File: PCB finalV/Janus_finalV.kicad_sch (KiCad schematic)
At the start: 37 parts, among them J1 Conn_01x02, J10 Conn_01x02, J11 Conn_01x04, J14 Conn_01x04, J15 Conn_01x04, J2 Conn_01x04, J3 BU33SD5WG-TR, J4 R-78B5.0-2.0, J5 Conn_01x03, J6 Conn_01x03, J7 Conn_ST_STDC14, J8 Conn_01x06, J9 Conn_01x02, U1 STM32L552CCTx

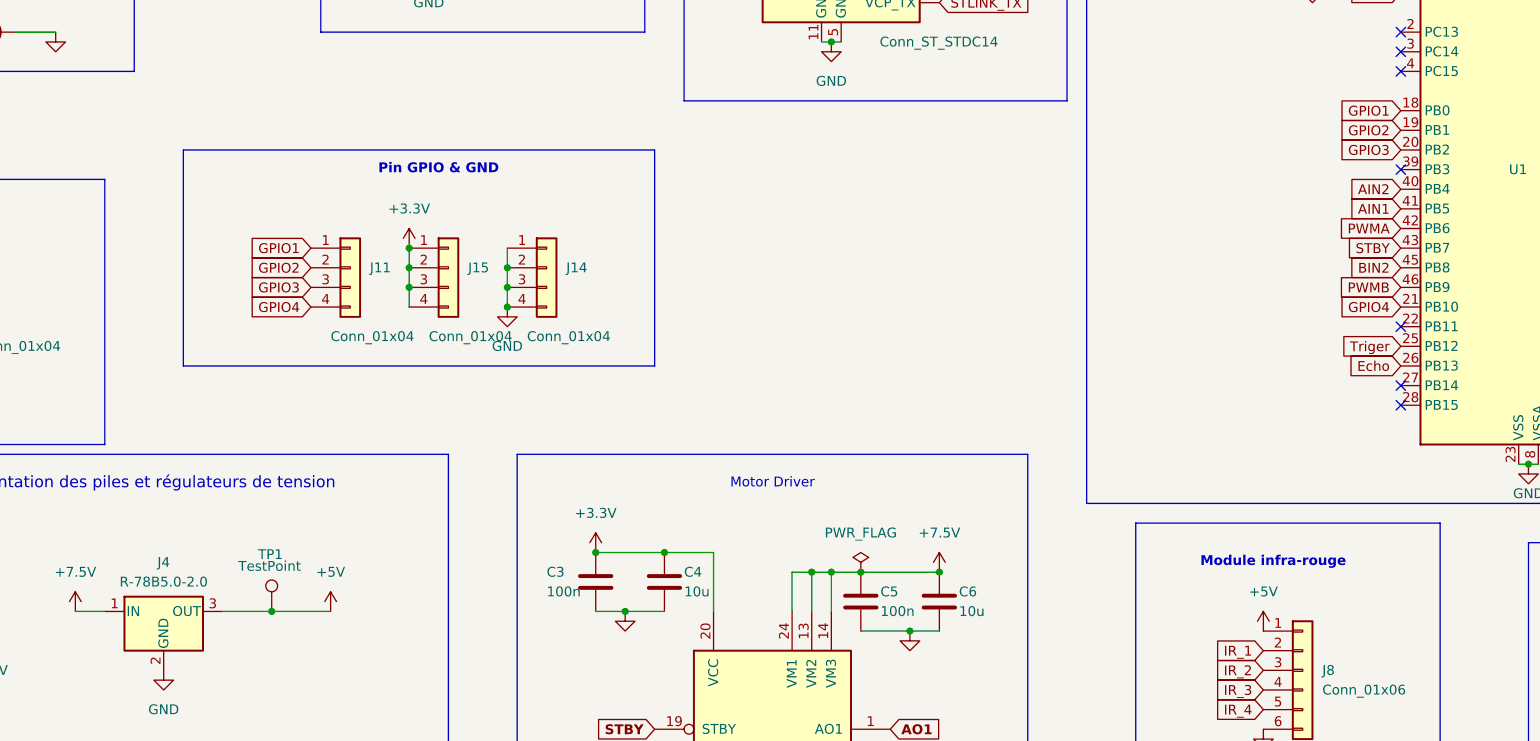
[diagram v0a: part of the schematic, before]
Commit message: MAJ code PAMI
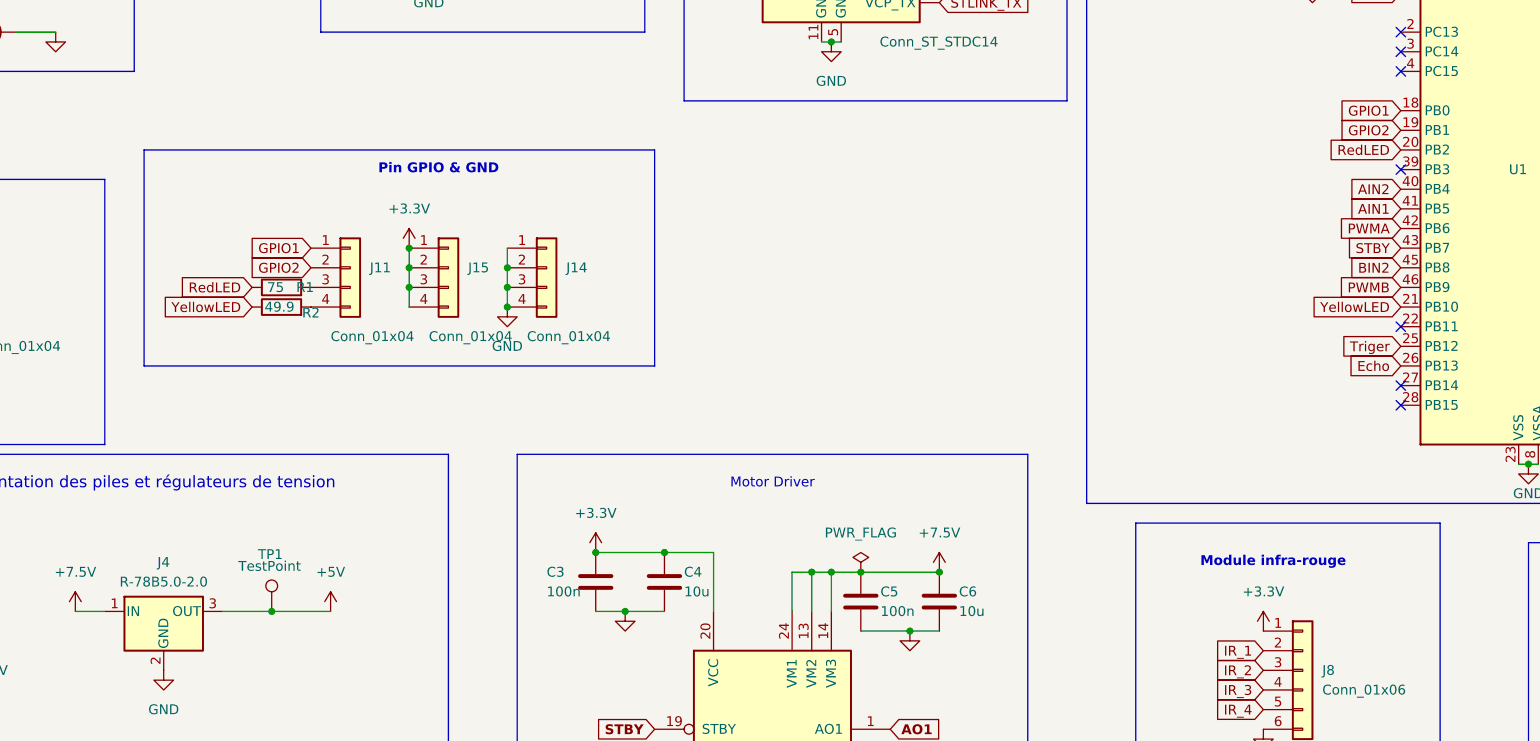
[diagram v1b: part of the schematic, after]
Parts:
- added R1: 75, Resistor_SMD:R_0402_1005Metric_Pad0.72x0.64mm_HandSolder, symbol Device:R
- added R2: 49.9, Resistor_SMD:R_0402_1005Metric_Pad0.72x0.64mm_HandSolder, symbol Device:R
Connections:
- net +3.3V: now also J8.1 (Pin_1)
- net +5V: no longer J8.1 (Pin_1)
- net GPIO3: no longer names the net of J11.3 (Pin_3)
- net GPIO3: now also R1.2; no longer U1.20 (PB2)
- net GPIO4: no longer names the net of J11.4 (Pin_4)
- net GPIO4: now also R2.2; no longer U1.21 (PB10)
- new net RedLED: R1.1, U1.20 (PB2)
- new net YellowLED: R2.1, U1.21 (PB10)
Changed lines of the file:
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@@
 		(date "2025-02-04")
 		(comment 1 "Capodagli Janus")
+		(comment 2 "REDLED 151051RS04000")
+		(comment 3 "YELLOWLED 151051YS04000")
 	)
 	(rectangle
@@
 	)
 	(rectangle
-		(start 66.04 76.2)
+		(start 60.96 76.2)
 		(end 127 104.14)
 		(stroke
@@
 		)
 	)
-	(global_label "GPIO3"
+	(global_label "RedLED"
 		(shape input)
 		(at 223.52 76.2 180)
@@
 		)
 		(property "Intersheetrefs" "${INTERSHEET_REFS}"
-			(at 214.85 76.2 0)
+			(at 213.5801 76.2 0)
 			(effects
 				(font
@@
 		)
 	)
-	(global_label "GPIO3"
+	(global_label "RedLED"
 		(shape input)
-		(at 82.55 93.98 180)
+		(at 74.93 93.98 180)
 		(fields_autoplaced yes)
 		(effects
@@
 		)
 		(property "Intersheetrefs" "${INTERSHEET_REFS}"
-			(at 73.88 93.98 0)
+			(at 64.9901 93.98 0)
 			(effects
 				(font
@@
 		)
 	)
-	(global_label "GPIO4"
+	(global_label "YellowLED"
 		(shape input)
 		(at 223.52 96.52 180)
@@
 		)
 		(property "Intersheetrefs" "${INTERSHEET_REFS}"
-			(at 214.85 96.52 0)
+			(at 211.1006 96.52 0)
 			(effects
 				(font
@@
 		)
 	)
-	(global_label "GPIO4"
+	(global_label "YellowLED"
 		(shape input)
-		(at 82.55 96.52 180)
+		(at 74.93 96.52 180)
 		(fields_autoplaced yes)
 		(effects
@@
 		)
 		(property "Intersheetrefs" "${INTERSHEET_REFS}"
-			(at 73.88 96.52 0)
+			(at 62.5106 96.52 0)
 			(effects
 				(font
@@
 	)
 	(symbol
+		(lib_id "Device:R")
+		(at 78.74 93.98 90)
+		(unit 1)
+		(exclude_from_sim no)
+		(in_bom yes)
+		(on_board yes)
+		(dnp no)
+		(property "Reference" "R1"
+			(at 81.788 93.98 90)
+			(effects
+				(font
+					(size 1.27 1.27)
+				)
+			)
+		)
+		(property "Value" "75"
+			(at 77.978 93.98 90)
+			(effects
+				(font
+					(size 1.27 1.27)
+				)
+			)
+		)
+		(property "Footprint" "Resistor_SMD:R_0402_1005Metric_Pad0.72x0.64mm_HandSolder"
+			(at 78.74 95.758 90)
+			(effects
+				(font
+					(size 1.27 1.27)
+				)
+				(hide yes)
+			)
+		)
+		(property "Datasheet" "560112110050"
+			(at 78.74 93.98 0)
+			(effects
+				(font
+					(size 1.27 1.27)
+				)
+				(hide yes)
+			)
+		)
+		(property "Description" "Resistor"
+			(at 78.74 93.98 0)
+			(effects
+				(font
+					(size 1.27 1.27)
+				)
+				(hide yes)
+			)
+		)
+		(pin "1"
+		)
+		(pin "2"
+		)
+		(instances
+			(project "Janus_finalV"
+				(path "/a7143e5e-39f3-42a3-a239-a1312258aecf"
+					(reference "R1")
+					(unit 1)
+				)
+			)
+		)
+	)
+	(symbol
 		(lib_id "power:GND")
 		(at 254 38.1 0)
@@
 	)
 	(symbol
+		(lib_id "power:+3.3V")
+		(at 205.74 138.43 0)
+		(unit 1)
+		(exclude_from_sim no)
+		(in_bom yes)
+		(on_board yes)
+		(dnp no)
+		(fields_autoplaced yes)
+		(property "Reference" "#PWR028"
+			(at 205.74 142.24 0)
+			(effects
+				(font
+					(size 1.27 1.27)
+				)
+				(hide yes)
+			)
+		)
+		(property "Value" "+3.3V"
+			(at 205.74 133.35 0)
+			(effects
+				(font
+					(size 1.27 1.27)
+				)
+			)
+		)
+		(property "Footprint" ""
+			(at 205.74 138.43 0)
+			(effects
+				(font
+					(size 1.27 1.27)
+				)
+				(hide yes)
+			)
+		)
+		(property "Datasheet" ""
+			(at 205.74 138.43 0)
+			(effects
+				(font
+					(size 1.27 1.27)
+				)
+				(hide yes)
+			)
+		)
+		(property "Description" "Power symbol creates a global label with name \"+3.3V\""
+			(at 205.74 138.43 0)
+			(effects
+				(font
+					(size 1.27 1.27)
+				)
+				(hide yes)
+			)
+		)
+		(pin "1"
+		)
+		(instances
+			(project "Janus_finalV"
+				(path "/a7143e5e-39f3-42a3-a239-a1312258aecf"
+					(reference "#PWR028")
+					(unit 1)
+				)
+			)
+		)
+	)
+	(symbol
 		(lib_name "GND_3")
 		(lib_id "power:GND")
@@
 	)
 	(symbol
-		(lib_id "power:+5V")
-		(at 205.74 138.43 0)
+		(lib_id "Device:R")
+		(at 78.74 96.52 90)
 		(unit 1)
 		(exclude_from_sim no)
@@
 		(on_board yes)
 		(dnp no)
-		(fields_autoplaced yes)
-		(property "Reference" "#PWR028"
-			(at 205.74 142.24 0)
+		(property "Reference" "R2"
+			(at 82.55 97.282 90)
 			(effects
 				(font
 					(size 1.27 1.27)
 				)
-				(hide yes)
 			)
 		)
-		(property "Value" "+5V"
-			(at 205.74 133.35 0)
+		(property "Value" "49.9"
+			(at 78.486 96.52 90)
 			(effects
 				(font
@@
 			)
 		)
-		(property "Footprint" ""
-			(at 205.74 138.43 0)
+		(property "Footprint" "Resistor_SMD:R_0402_1005Metric_Pad0.72x0.64mm_HandSolder"
+			(at 78.74 98.298 90)
 			(effects
 				(font
@@
 			)
 		)
-		(property "Datasheet" ""
-			(at 205.74 138.43 0)
+		(property "Datasheet" "560112110002"
+			(at 78.74 96.52 0)
 			(effects
 				(font
@@
 			)
 		)
-		(property "Description" "Power symbol creates a global label with name \"+5V\""
-			(at 205.74 138.43 0)
+		(property "Description" "Resistor"
+			(at 78.74 96.52 0)
 			(effects
 				(font
@@
 		(pin "1"
 		)
+		(pin "2"
+		)
 		(instances
-			(project ""
+			(project "Janus_finalV"
 				(path "/a7143e5e-39f3-42a3-a239-a1312258aecf"
-					(reference "#PWR028")
+					(reference "R2")
 					(unit 1)
 				)
